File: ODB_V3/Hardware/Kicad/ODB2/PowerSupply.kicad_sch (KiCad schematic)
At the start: 53 parts, among them J15 Vin_XT30PW-F, U13 L6981N33DR, U7 MPQ9843GLE-5-AEC1-Z

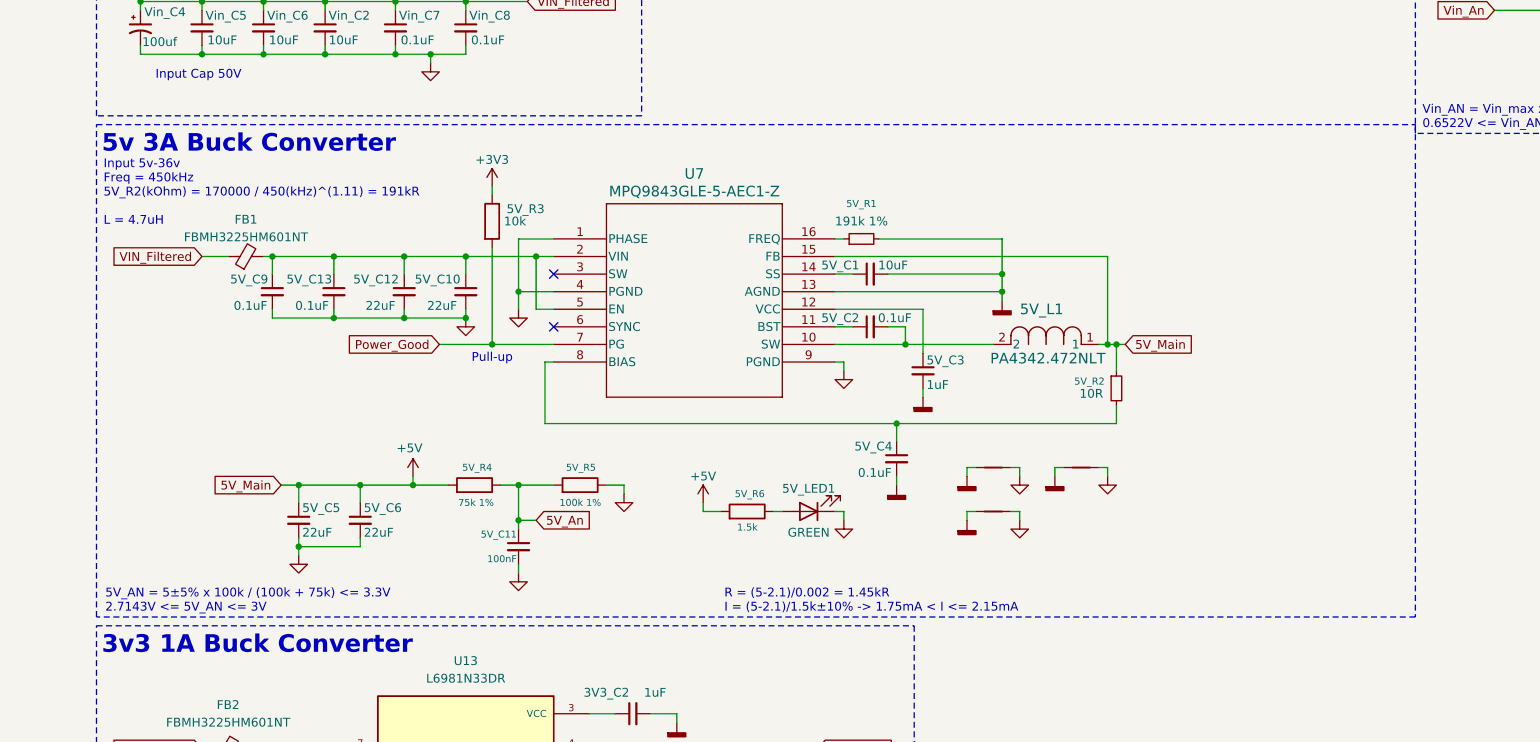
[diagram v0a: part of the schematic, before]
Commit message: wip: pyro trace
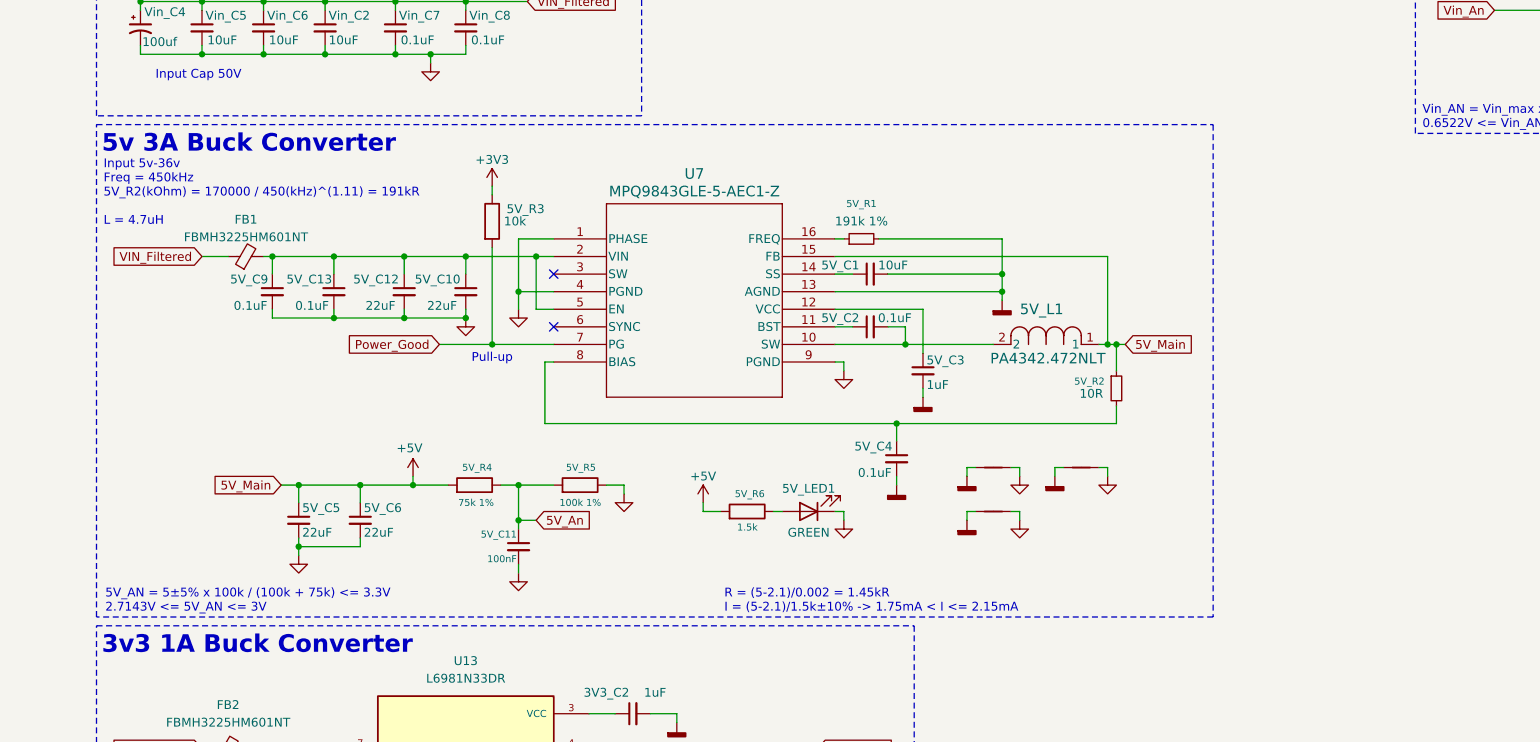
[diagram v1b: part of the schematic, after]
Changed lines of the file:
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@@
 	(rectangle
 		(start 15.24 52.07)
-		(end 205.74 123.19)
+		(end 176.53 123.19)
 		(stroke
 			(width 0)
